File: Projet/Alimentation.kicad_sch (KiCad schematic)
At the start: 12 parts, among them J501 alim batterie, J502 Conn_01x03_Female, U501 AZ1117-5.0, U502 MIC5317-3.3

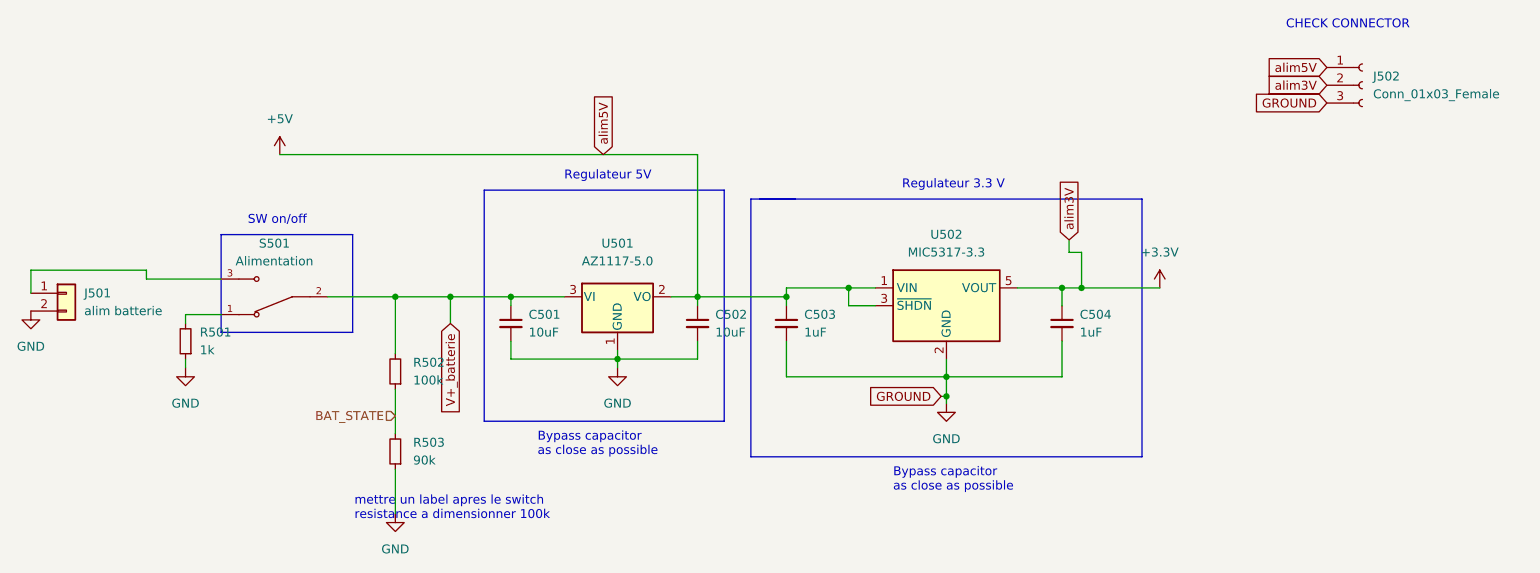
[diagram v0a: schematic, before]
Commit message: placement
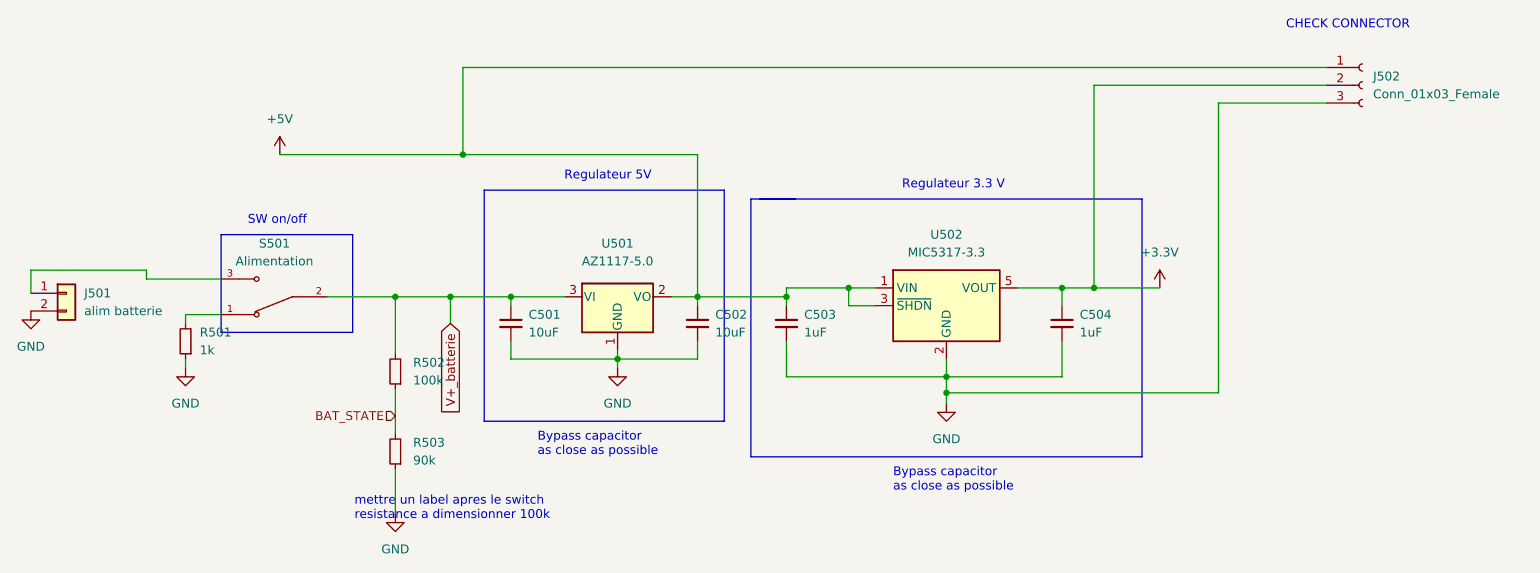
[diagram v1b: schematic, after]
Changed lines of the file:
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@@
   (junction (at 128.27 87.63) (diameter 0) (color 0 0 0 0)
   )
+  (junction (at 163.83 101.346) (diameter 0) (color 0 0 0 0)
+  )
   (junction (at 163.83 99.06) (diameter 0) (color 0 0 0 0)
   )
@@
   (junction (at 101.6 87.63) (diameter 0) (color 0 0 0 0)
   )
-  (junction (at 163.83 101.854) (diameter 0) (color 0 0 0 0)
-  )
-  (junction (at 183.134 86.36) (diameter 0) (color 0 0 0 0)
+  (junction (at 184.912 86.36) (diameter 0) (color 0 0 0 0)
   )
   (junction (at 92.964 87.63) (diameter 0) (color 0 0 0 0)
@@
   (junction (at 180.34 86.36) (diameter 0) (color 0 0 0 0)
   )
+  (junction (at 94.742 67.31) (diameter 0) (color 0 0 0 0)
+  )
   (junction (at 149.86 86.36) (diameter 0) (color 0 0 0 0)
   )
@@
     (stroke (width 0) (type default) (color 0 0 0 0))
   )
-  (wire (pts (xy 181.356 79.502) (xy 181.356 81.28))
-    (stroke (width 0) (type default) (color 0 0 0 0))
-  )
   (wire (pts (xy 128.27 87.63) (xy 140.97 87.63))
     (stroke (width 0) (type default) (color 0 0 0 0))
@@
     (stroke (width 0) (type default) (color 0 0 0 0))
   )
+  (wire (pts (xy 202.692 101.346) (xy 163.83 101.346))
+    (stroke (width 0) (type default) (color 0 0 0 0))
+  )
   (polyline (pts (xy 191.77 110.49) (xy 135.89 110.49))
     (stroke (width 0) (type default) (color 0 0 0 0))
   )
+  (wire (pts (xy 218.186 57.404) (xy 184.912 57.404))
+    (stroke (width 0) (type default) (color 0 0 0 0))
+  )
   (wire (pts (xy 85.09 100.838) (xy 85.09 107.188))
     (stroke (width 0) (type default) (color 0 0 0 0))
@@
     (stroke (width 0) (type default) (color 0 0 0 0))
   )
+  (wire (pts (xy 94.742 54.864) (xy 94.742 67.31))
+    (stroke (width 0) (type default) (color 0 0 0 0))
+  )
   (wire (pts (xy 55.118 90.17) (xy 60.198 90.17))
     (stroke (width 0) (type default) (color 0 0 0 0))
@@
     (stroke (width 0) (type default) (color 0 0 0 0))
   )
+  (wire (pts (xy 218.186 54.864) (xy 94.742 54.864))
+    (stroke (width 0) (type default) (color 0 0 0 0))
+  )
   (polyline (pts (xy 60.198 78.74) (xy 60.198 92.71))
     (stroke (width 0) (type default) (color 0 0 0 0))
@@
     (stroke (width 0) (type default) (color 0 0 0 0))
   )
-  (wire (pts (xy 163.83 99.06) (xy 163.83 101.854))
+  (wire (pts (xy 163.83 99.06) (xy 163.83 101.346))
+    (stroke (width 0) (type default) (color 0 0 0 0))
+  )
+  (wire (pts (xy 202.692 59.944) (xy 202.692 101.346))
     (stroke (width 0) (type default) (color 0 0 0 0))
   )
@@
     (stroke (width 0) (type default) (color 0 0 0 0))
   )
-  (wire (pts (xy 163.83 101.854) (xy 163.83 102.87))
-    (stroke (width 0) (type default) (color 0 0 0 0))
-  )
   (wire (pts (xy 85.09 95.758) (xy 85.09 87.63))
     (stroke (width 0) (type default) (color 0 0 0 0))
@@
     (stroke (width 0) (type default) (color 0 0 0 0))
   )
-  (wire (pts (xy 68.58 67.31) (xy 128.27 67.31))
+  (wire (pts (xy 68.58 67.31) (xy 94.742 67.31))
     (stroke (width 0) (type default) (color 0 0 0 0))
   )
@@
     (stroke (width 0) (type default) (color 0 0 0 0))
   )
-  (wire (pts (xy 180.34 86.36) (xy 183.134 86.36))
-    (stroke (width 0) (type default) (color 0 0 0 0))
-  )
   (wire (pts (xy 55.118 96.52) (xy 55.118 97.79))
     (stroke (width 0) (type default) (color 0 0 0 0))
@@
     (stroke (width 0) (type default) (color 0 0 0 0))
   )
+  (wire (pts (xy 163.83 101.346) (xy 163.83 102.87))
+    (stroke (width 0) (type default) (color 0 0 0 0))
+  )
+  (wire (pts (xy 94.742 67.31) (xy 128.27 67.31))
+    (stroke (width 0) (type default) (color 0 0 0 0))
+  )
   (wire (pts (xy 153.67 86.36) (xy 149.86 86.36))
     (stroke (width 0) (type default) (color 0 0 0 0))
@@
     (stroke (width 0) (type default) (color 0 0 0 0))
   )
-  (wire (pts (xy 181.356 81.28) (xy 183.134 81.28))
-    (stroke (width 0) (type default) (color 0 0 0 0))
-  )
   (wire (pts (xy 33.02 83.82) (xy 33.02 87.122))
     (stroke (width 0) (type default) (color 0 0 0 0))
@@
     (stroke (width 0) (type default) (color 0 0 0 0))
   )
-  (wire (pts (xy 183.134 81.28) (xy 183.134 86.36))
+  (wire (pts (xy 184.912 57.404) (xy 184.912 86.36))
+    (stroke (width 0) (type default) (color 0 0 0 0))
+  )
+  (wire (pts (xy 184.912 86.36) (xy 194.31 86.36))
     (stroke (width 0) (type default) (color 0 0 0 0))
   )
@@
     (stroke (width 0) (type default) (color 0 0 0 0))
   )
-  (wire (pts (xy 163.068 101.854) (xy 163.83 101.854))
-    (stroke (width 0) (type default) (color 0 0 0 0))
-  )
-  (wire (pts (xy 183.134 86.36) (xy 194.31 86.36))
+  (wire (pts (xy 180.34 86.36) (xy 184.912 86.36))
     (stroke (width 0) (type default) (color 0 0 0 0))
   )
   (wire (pts (xy 101.6 87.63) (xy 101.6 88.9))
+    (stroke (width 0) (type default) (color 0 0 0 0))
+  )
+  (wire (pts (xy 218.186 59.944) (xy 202.692 59.944))
     (stroke (width 0) (type default) (color 0 0 0 0))
   )
@@
       (effects (font (size 1.27 1.27)) (justify right) hide)
     )
-  )
-  (global_label "alim5V" (shape input) (at 114.808 67.31 90) (fields_autoplaced)
-    (effects (font (size 1.27 1.27)) (justify left))
-    (property "Intersheet References" "${INTERSHEET_REFS}" (id 0) (at 114.7286 58.4864 90)
-      (effects (font (size 1.27 1.27)) (justify left) hide)
-    )
-  )
-  (global_label "GROUND" (shape input) (at 163.068 101.854 180) (fields_autoplaced)
-    (effects (font (size 1.27 1.27)) (justify right))
-    (property "Intersheet References" "${INTERSHEET_REFS}" (id 0) (at 152.8535 101.9334 0)
-      (effects (font (size 1.27 1.27)) (justify right) hide)
-    )
-  )
-  (global_label "GROUND" (shape input) (at 218.186 59.944 180) (fields_autoplaced)
-    (effects (font (size 1.27 1.27)) (justify right))
-    (property "Intersheet References" "${INTERSHEET_REFS}" (id 0) (at 207.9715 60.0234 0)
-      (effects (font (size 1.27 1.27)) (justify right) hide)
-    )
-  )
-  (global_label "alim3V" (shape input) (at 181.356 79.502 90) (fields_autoplaced)
-    (effects (font (size 1.27 1.27)) (justify left))
-    (property "Intersheet References" "${INTERSHEET_REFS}" (id 0) (at 181.2766 70.6784 90)
-      (effects (font (size 1.27 1.27)) (justify left) hide)
-    )
-  )
-  (global_label "alim3V" (shape input) (at 218.186 57.404 180) (fields_autoplaced)
-    (effects (font (size 1.27 1.27)) (justify right))
-    (property "Intersheet References" "${INTERSHEET_REFS}" (id 0) (at 209.3624 57.4834 0)
-      (effects (font (size 1.27 1.27)) (justify right) hide)
-    )
-  )
-  (global_label "alim5V" (shape input) (at 218.186 54.864 180) (fields_autoplaced)
-    (effects (font (size 1.27 1.27)) (justify right))
-    (property "Intersheet References" "${INTERSHEET_REFS}" (id 0) (at 209.3624 54.9434 0)
-      (effects (font (size 1.27 1.27)) (justify right) hide)
-    )
